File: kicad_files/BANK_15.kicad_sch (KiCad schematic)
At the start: 1 part, among them IC1 XC7S25-1CSGA225C

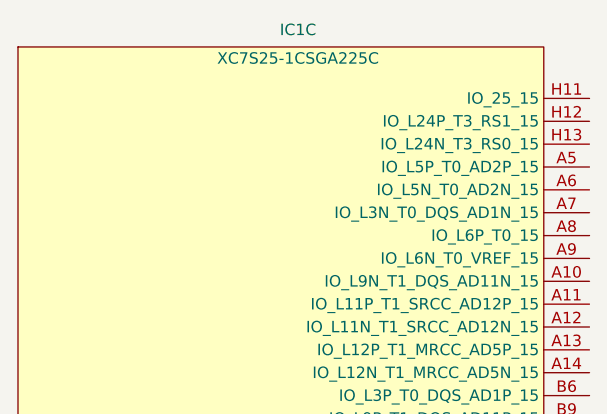
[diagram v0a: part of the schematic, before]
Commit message: schematic updated
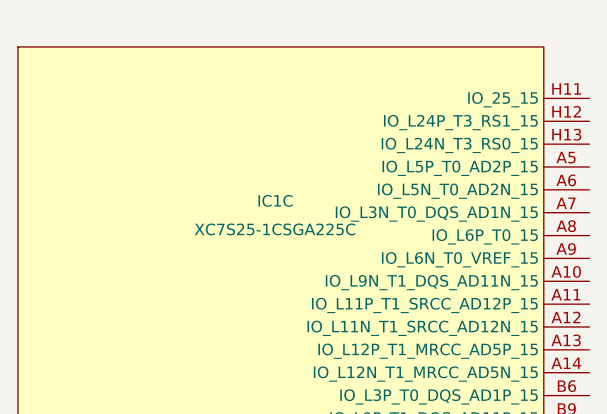
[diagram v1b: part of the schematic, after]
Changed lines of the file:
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@@
   (symbol (lib_id "SamacSys_Parts:XC7S25-1CSGA225C") (at 105.41 109.855 0) (unit 3)
     (in_bom yes) (on_board yes) (dnp no)
-    (property "Reference" "IC1" (at 105.41 33.02 0)
+    (property "Reference" "IC1" (at 102.87 52.07 0)
       (effects (font (size 1.27 1.27)))
     )
-    (property "Value" "XC7S25-1CSGA225C" (at 105.41 36.195 0)
+    (property "Value" "XC7S25-1CSGA225C" (at 102.87 55.245 0)
       (effects (font (size 1.27 1.27)))
     )
@@
     (pin "R1")
     (pin "R15")
-    (pin "E5")
-    (pin "F5")
-    (pin "G5")
-    (pin "G8")
-    (pin "G9")
-    (pin "H14")
-    (pin "H15")
-    (pin "H5")
-    (pin "H8")
-    (pin "H9")
     (pin "J11")
-    (pin "J12")
     (pin "J15")
-    (pin "J5")
-    (pin "J8")
-    (pin "J9")
-    (pin "K11")
-    (pin "K12")
-    (pin "K13")
     (pin "K14")
     (pin "K15")
-    (pin "K4")
-    (pin "K5")
     (pin "L10")
-    (pin "L11")
     (pin "L12")
     (pin "L13")
     (pin "L14")
     (pin "L15")
-    (pin "L4")
-    (pin "L5")
     (pin "M10")
     (pin "M13")
     (pin "M14")
     (pin "M15")
-    (pin "M5")
-    (pin "M6")
     (pin "M7")
     (pin "M8")
     (pin "M9")
-    (pin "N10")
-    (pin "N11")
     (pin "N12")
     (pin "N13")
     (pin "N14")
     (pin "N15")
-    (pin "N5")
     (pin "N6")
     (pin "N7")
     (pin "N8")
     (pin "N9")
-    (pin "P10")
     (pin "P11")
     (pin "P12")
@@
           (reference "IC1") (unit 3)
         )
+        (path "/94bd3a84-5526-4cf2-a5cc-3887356f447c/30d52c37-ae5c-405e-8a78-89b18a6efc4e/af489dd5-0e9e-4b3e-a401-f1288bd8b210"
+          (reference "IC1") (unit 3)
+        )

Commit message: schematic updated
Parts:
- IC1: footprint BGA225C80P15X15_1300X1300X140 -> SamacSys_Parts:BGA225C80P15X15_1300X1300X140
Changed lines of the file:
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@@
       (effects (font (size 1.27 1.27)))
     )
-    (property "Footprint" "BGA225C80P15X15_1300X1300X140" (at 213.995 82.55 0)
+    (property "Footprint" "SamacSys_Parts:BGA225C80P15X15_1300X1300X140" (at 213.995 82.55 0)
       (effects (font (size 1.27 1.27)) (justify left top) hide)
     )
